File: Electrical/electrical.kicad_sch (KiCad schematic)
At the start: 14 parts, among them M1 Motor_DC, M2 Motor_DC, SW1 SW_Push, SW2 SW_Push, SW3 SW_DPST_x2, U1 MPXA6115A, U2 L298N

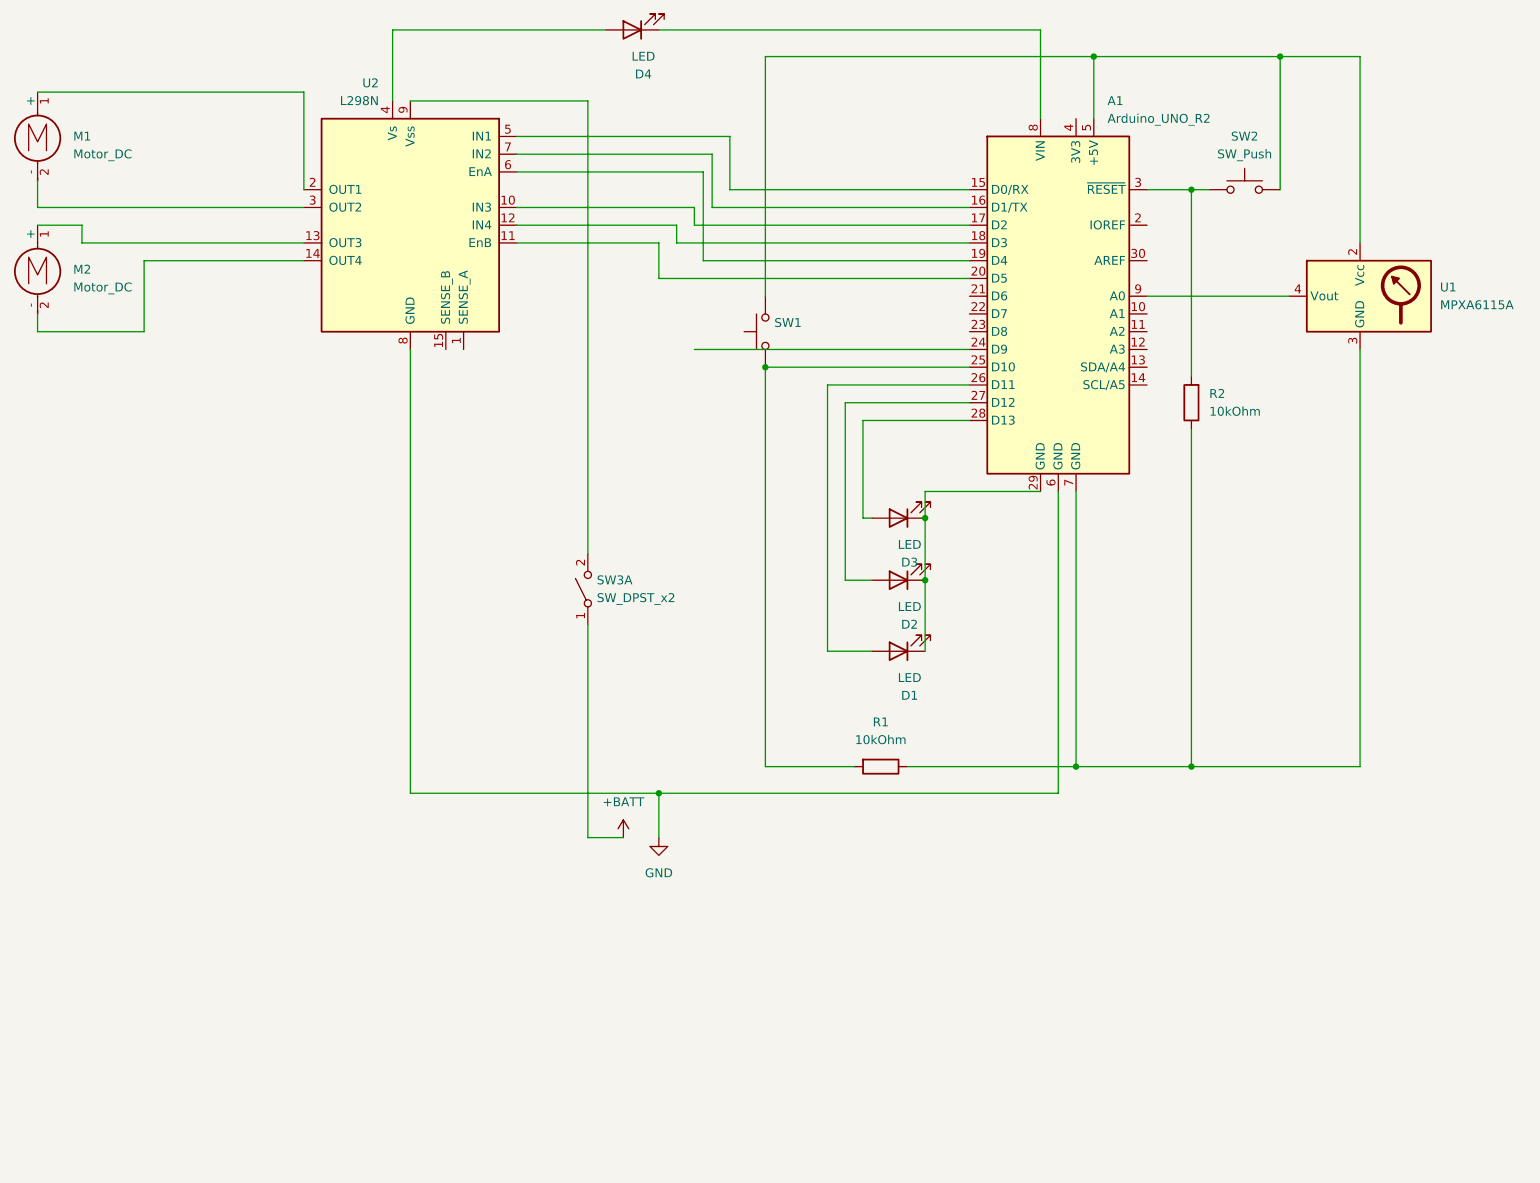
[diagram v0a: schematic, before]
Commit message: Konverting to Pico
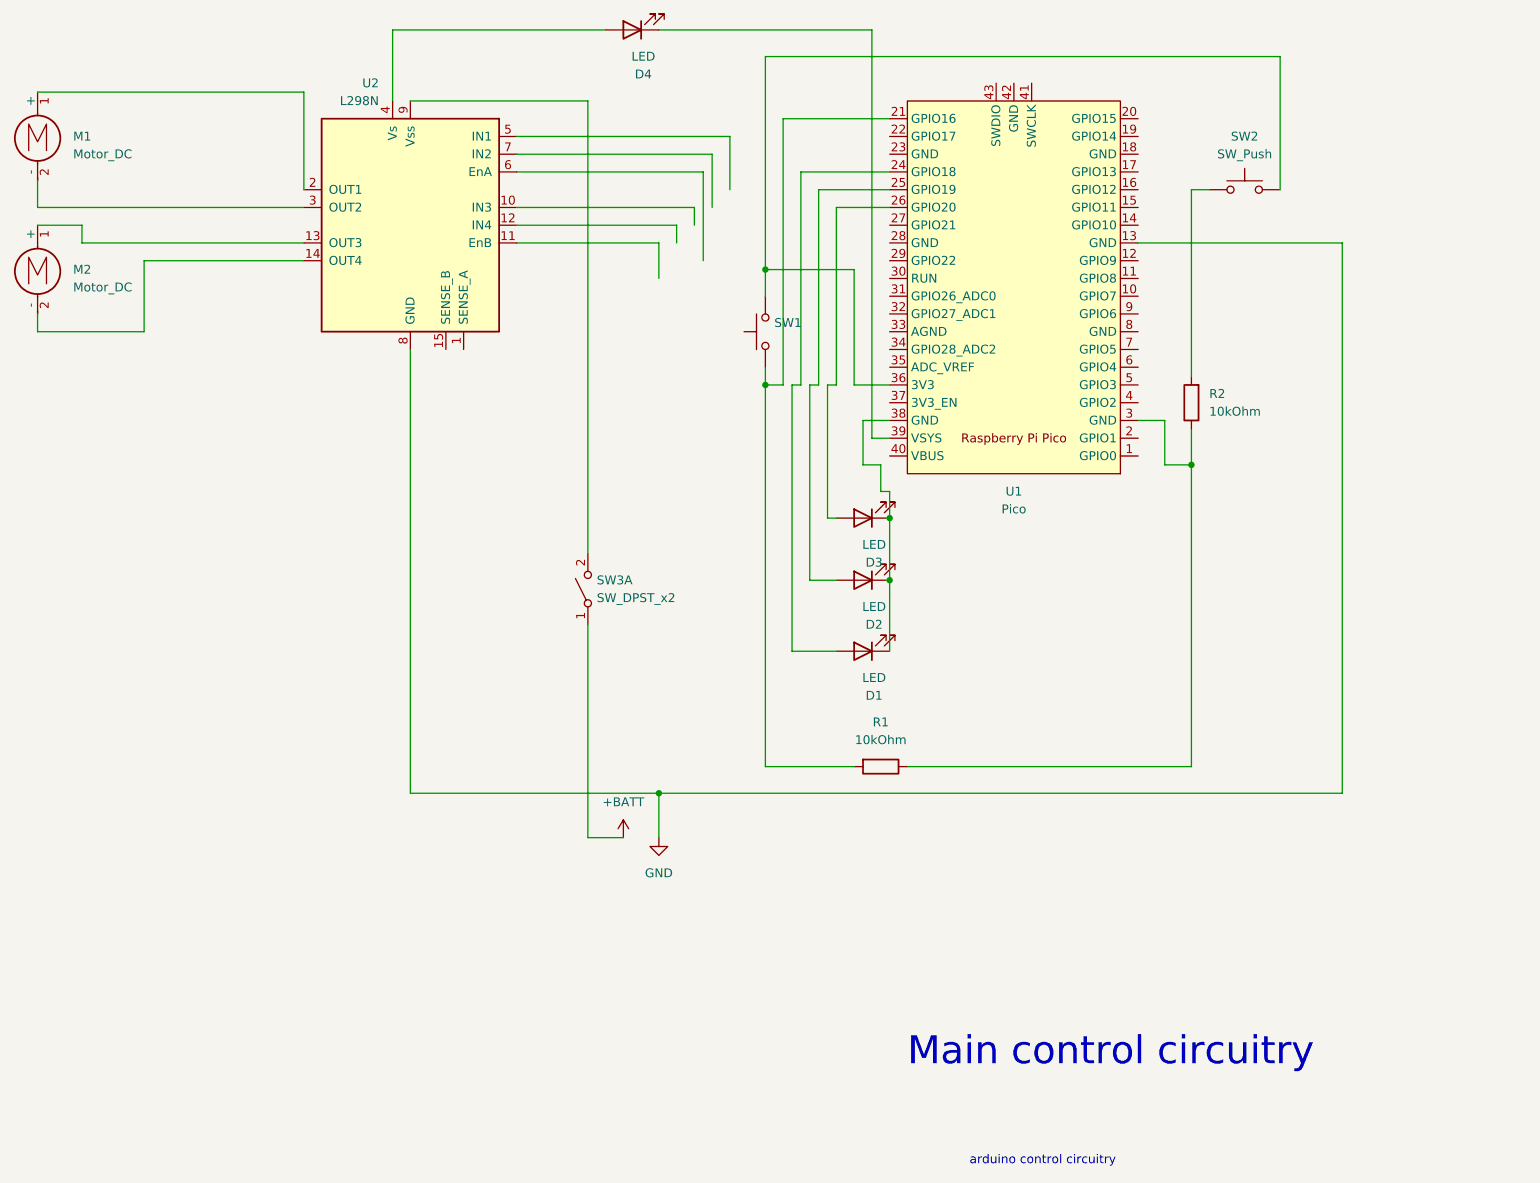
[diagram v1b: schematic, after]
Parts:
- removed A1: Arduino_UNO_R2, Module:Arduino_UNO_R2, symbol MCU_Module:Arduino_UNO_R2
- removed U1: MPXA6115A, symbol Sensor_Pressure:MPXA6115A
- added U1: Pico, RPi_Pico:RPi_Pico_SMD_TH, symbol MCU_RaspberryPi_and_Boards:Pico
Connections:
- net GND: now also U1.13 (GND)
- net at R1.1, R2.1: now also U1.3 (GND)
- net at D1.1 (K), D2.1 (K), D3.1 (K): now also U1.38 (GND)
- net at D3.2 (A): now also U1.26 (GPIO20)
- net at SW1.2, SW2.2: now also U1.36 (3V3)
- net at R1.2, SW1.1: now also U1.21 (GPIO16)
- net at D1.2 (A): now also U1.24 (GPIO18)
- net at D2.2 (A): now also U1.25 (GPIO19)
- net at D4.1 (K): now also U1.39 (VSYS)
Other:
- note added: "Main control circuitry"
- note added: "arduino control circuitry"
- moved on the sheet: D1, D2, D3
